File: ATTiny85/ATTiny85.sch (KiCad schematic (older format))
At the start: 21 parts, among them J2 Conn_01x05, J3 Conn_01x05, J4 ISP6, SW1 SW_SPST, U1 ATtiny85-20SU

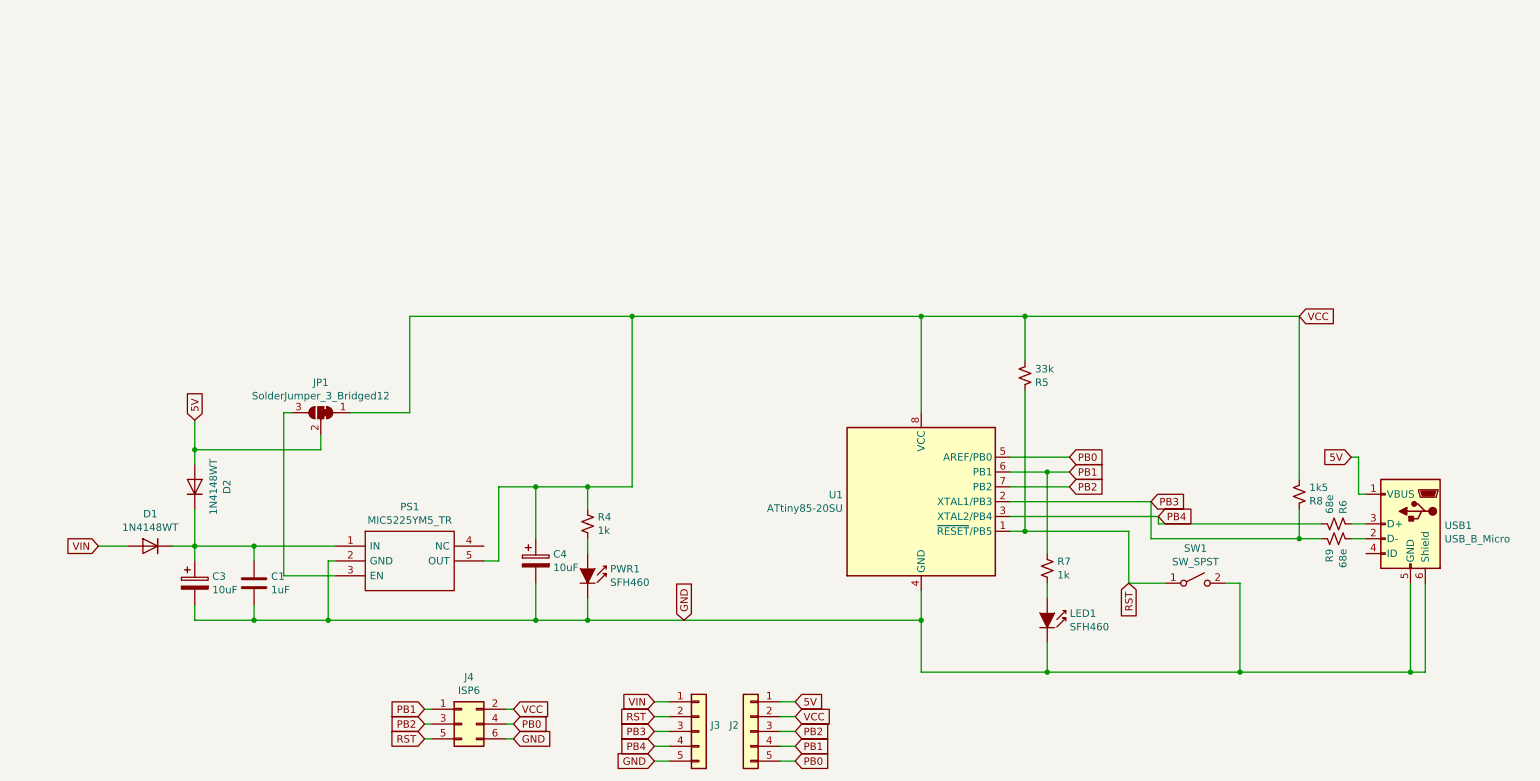
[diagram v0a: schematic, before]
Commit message: Schematic PDF and 3D Renders added
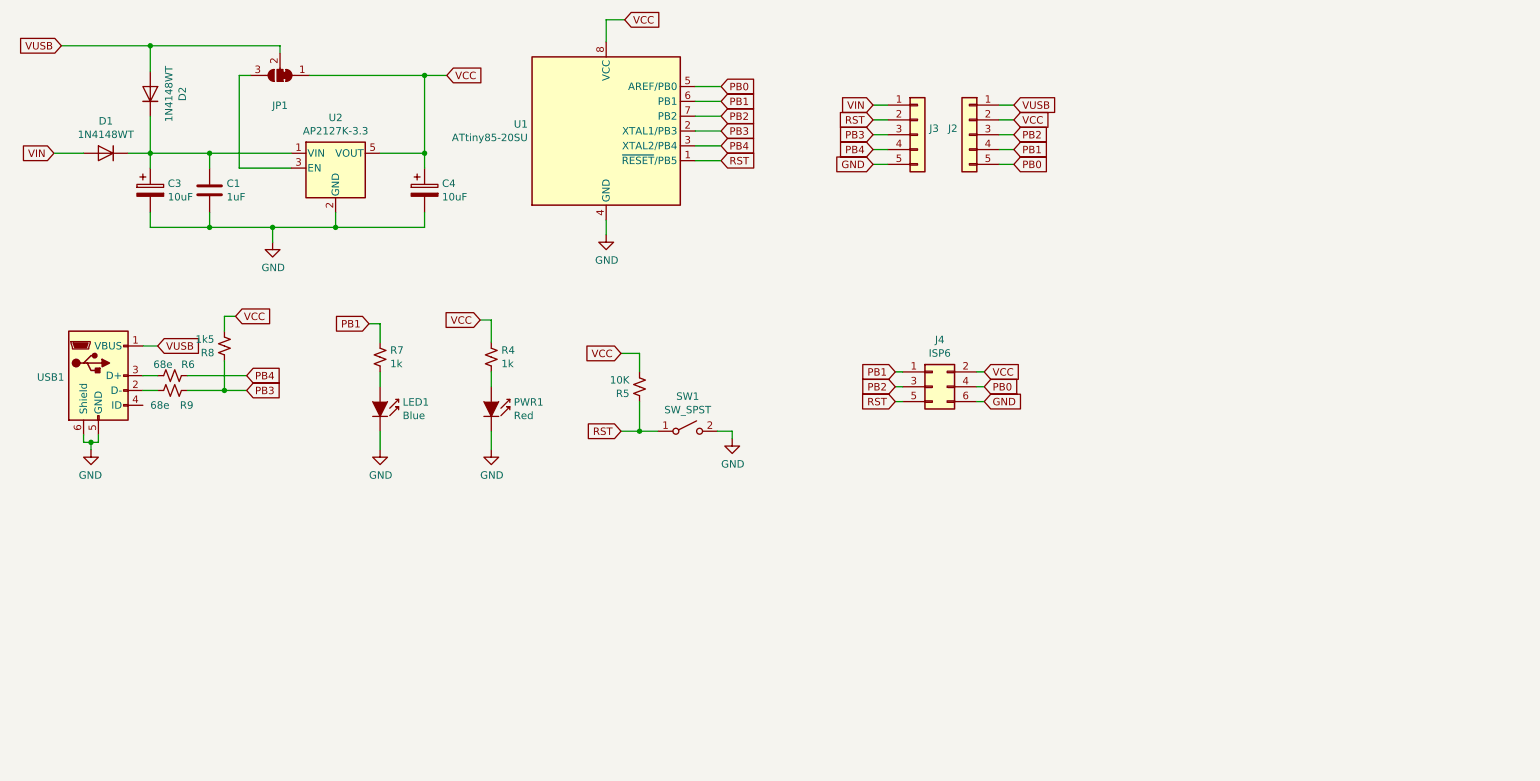
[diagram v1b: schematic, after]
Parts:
- removed PS1: MIC5225YM5_TR, SOT95P280X145-5N, symbol Adjustable_150mA_Regulator:MIC5225YM5_TR
- added U2: AP2127K-3.3, Package_TO_SOT_SMD:SOT-23-5, symbol Regulator_Linear:AP2127K-3.3
- C1: Part (none) -> C29936
- C3, C4: Part (none) -> C95841
- D1, D2: Part (none) -> C232841
- LED1: value SFH460 -> Blue; Part (none) -> C193191
- PWR1: value SFH460 -> Red; Part (none) -> C118330
- R4, R7: Part (none) -> C25585
- R5: value 33k -> 10K; Part (none) -> C99198
- R6, R9: Part (none) -> C325751
- R8: Part (none) -> C114668
- SW1: Part (none) -> C231329
- U1: Part (none) -> 177-2968
- USB1: Part (none) -> C132560
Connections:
- net GND: now also U2.2 (GND)
- net VCC: now also U2.5 (VOUT)
- net at C1.1, C3.1, D1.1 (K)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: now also U2.1 (VIN)
- net at JP1.3 (B): now also U2.3 (EN)
- net 5V renamed VUSB
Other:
- moved on the sheet: C1, C3, C4, D1, D2, J2, J3, J4, JP1, LED1, PWR1, R4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
